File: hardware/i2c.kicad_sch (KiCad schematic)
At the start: 21 parts, among them Q2 SS8550, Q3 SS8050, U11 SAINTCON-Minibadge, U12 SAINTCON-Minibadge, U3 SAINTCON-Minibadge, U4 SAINTCON-Minibadge, U5 SAINTCON-Minibadge, U6 SAINTCON-Minibadge, U8 SAINTCON-Minibadge, U9 SAINTCON-Minibadge

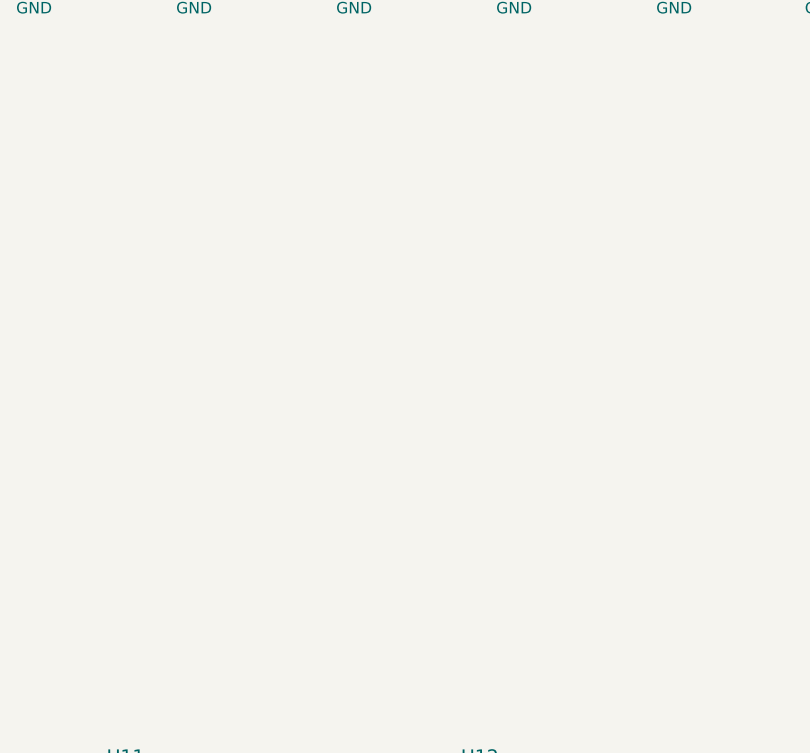
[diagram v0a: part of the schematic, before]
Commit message: accel added
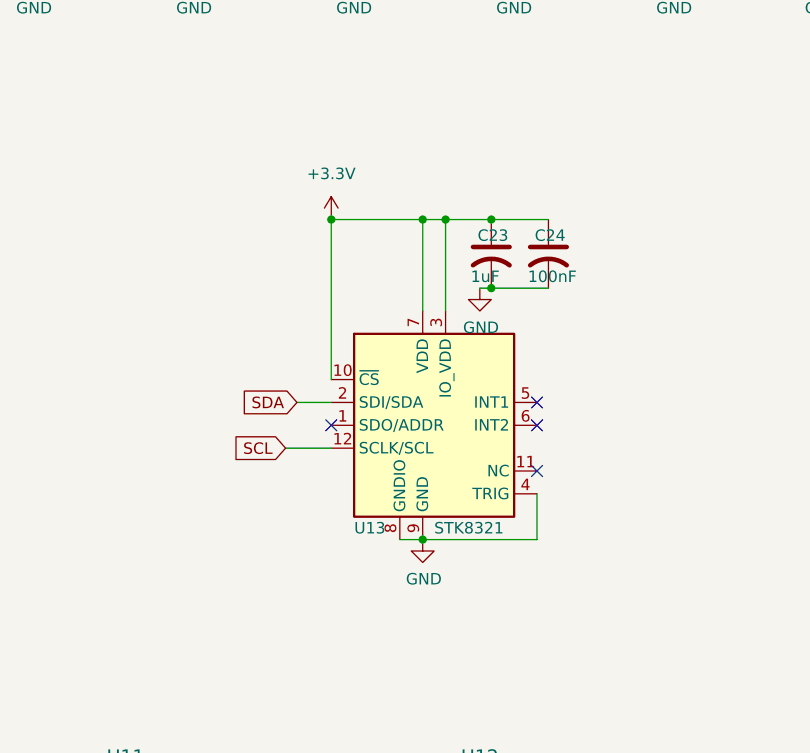
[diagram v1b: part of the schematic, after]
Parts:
- added C23: 1uF, C_0603_1608Metric, symbol Device:C_US
- added C24: 100nF, C_0603_1608Metric, symbol Device:C_US
- added U13: STK8321, Package_LGA:LGA-12_2x2mm_P0.5mm, symbol Sensor_Motion:KX022-1020
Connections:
- net +3.3V: now also C23.1, C24.1, U13.10 (~{CS}), U13.3 (IO_VDD), U13.7 (VDD)
- net GND: now also C23.2, C24.2, U13.4 (TRIG), U13.8 (GNDIO), U13.9 (GND)
- net SCL: now also U13.12 (SCLK/SCL)
- net SDA: now also U13.2 (SDI/SDA)
- no-connect marks 33 -> 37
